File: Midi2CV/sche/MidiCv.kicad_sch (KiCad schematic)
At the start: 41 parts, among them Q1 2N7000, Q2 2N7000, Q3 2N7000, Q4 2N7000, Q5 2N7000, Q6 2N7000, Q7 2N7000, Q8 2N7000, U1 STM32F103C8T6_BD, U2 6N138

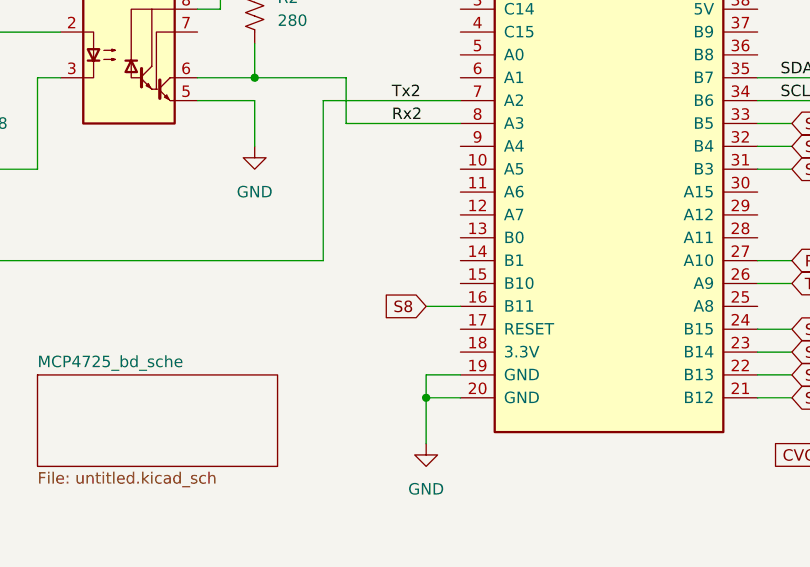
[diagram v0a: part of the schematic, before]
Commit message: update midi2cv schematic
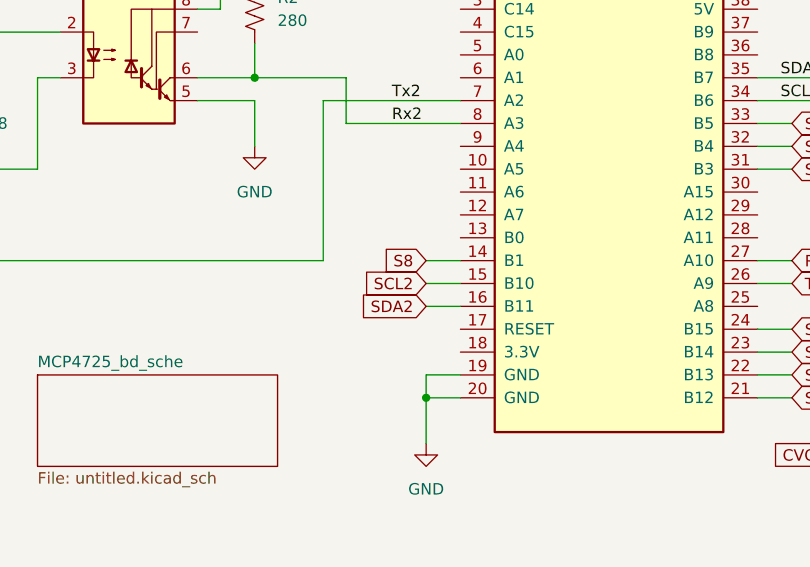
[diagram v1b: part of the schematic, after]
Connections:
- net S8: now also U1.14 (B1); no longer U1.16 (B11)
- net SCL2: now reaches U1.15 (B10)
- new net SDA2: U1.16 (B11)
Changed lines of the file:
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@@
+    (stroke (width 0) (type default))
+  )
+  (wire (pts (xy 107.95 71.12) (xy 111.76 71.12))
     (stroke (width 0) (type default))
   )
@@
     (stroke (width 0) (type default))
   )
+  (wire (pts (xy 107.95 66.04) (xy 111.76 66.04))
+    (stroke (width 0) (type default))
+  )
   (wire (pts (xy 226.06 29.21) (xy 226.06 48.26))
     (stroke (width 0) (type default))
@@
     (stroke (width 0) (type default))
   )
-  (wire (pts (xy 107.95 71.12) (xy 111.76 71.12))
-    (stroke (width 0) (type default))
-  )
   (wire (pts (xy 19.05 55.88) (xy 52.07 55.88))
     (stroke (width 0) (type default))
@@
   )
   (wire (pts (xy 88.9 45.72) (xy 99.06 45.72))
+    (stroke (width 0) (type default))
+  )
+  (wire (pts (xy 107.95 68.58) (xy 111.76 68.58))
     (stroke (width 0) (type default))
   )
@@
     )
   )
-  (global_label "S8" (shape input) (at 107.95 71.12 180) (fields_autoplaced)
-    (effects (font (size 1.27 1.27)) (justify right))
-    (property "Intersheetrefs" "${INTERSHEET_REFS}" (at 102.5458 71.12 0)
+  (global_label "S8" (shape input) (at 107.95 66.04 180) (fields_autoplaced)
+    (effects (font (size 1.27 1.27)) (justify right))
+    (property "Intersheetrefs" "${INTERSHEET_REFS}" (at 102.5458 66.04 0)
       (effects (font (size 1.27 1.27)) (justify right) hide)
     )
@@
     )
   )
+  (global_label "SCL2" (shape input) (at 107.95 68.58 180) (fields_autoplaced)
+    (effects (font (size 1.27 1.27)) (justify right))
+    (property "Intersheetrefs" "${INTERSHEET_REFS}" (at 100.2477 68.58 0)
+      (effects (font (size 1.27 1.27)) (justify right) hide)
+    )
+  )
   (global_label "S8" (shape input) (at 267.97 109.22 0) (fields_autoplaced)
     (effects (font (size 1.27 1.27)) (justify left))
@@
       (effects (font (size 1.27 1.27)) (justify right) hide)
     )
+  )
+  (global_label "SDA2" (shape input) (at 107.95 71.12 180) (fields_autoplaced)
+    (effects (font (size 1.27 1.27)) (justify right))
+    (property "Intersheetrefs" "${INTERSHEET_REFS}" (at 100.1872 71.12 0)
+      (effects (font (size 1.27 1.27)) (justify right) hide)
+    )
